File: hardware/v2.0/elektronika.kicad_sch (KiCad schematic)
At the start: 42 parts, among them J1 Conn_02x06_Odd_Even, J12 Conn_01x02, J2 Micro_SD_Card, J3 Conn_01x06, Q4 Q_NMOS_GSD, Q5 Q_PMOS_GSD, Q6 Q_NMOS_GSD, Q7 Q_NMOS_GSD, Q8 Q_NMOS_GSD

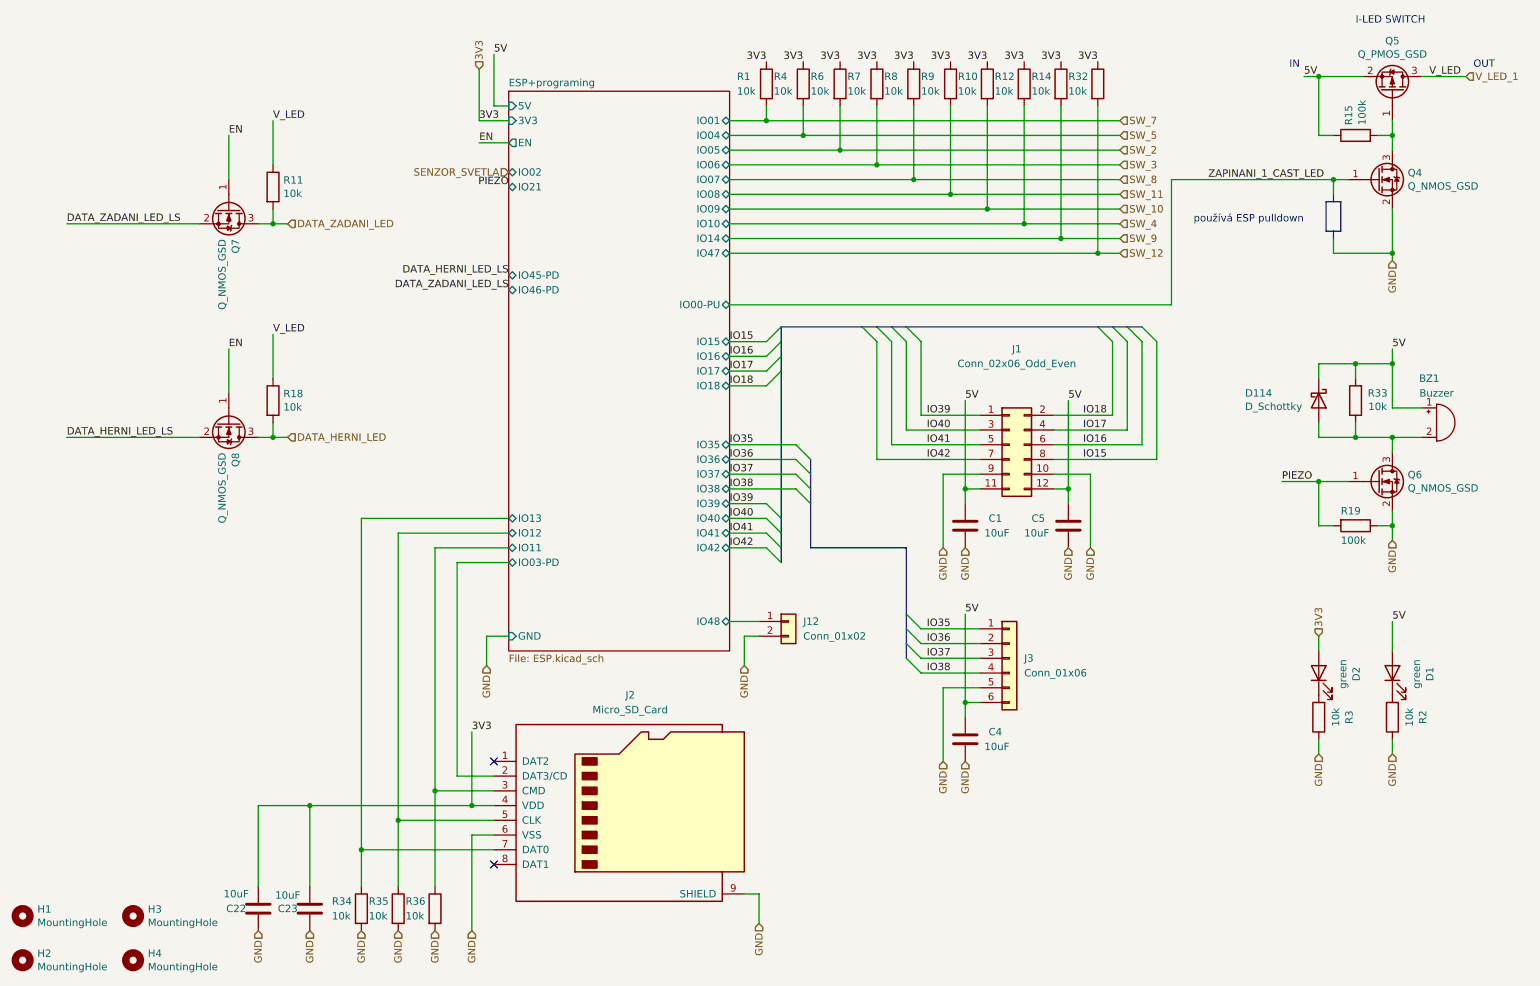
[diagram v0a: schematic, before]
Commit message: RH v2 version
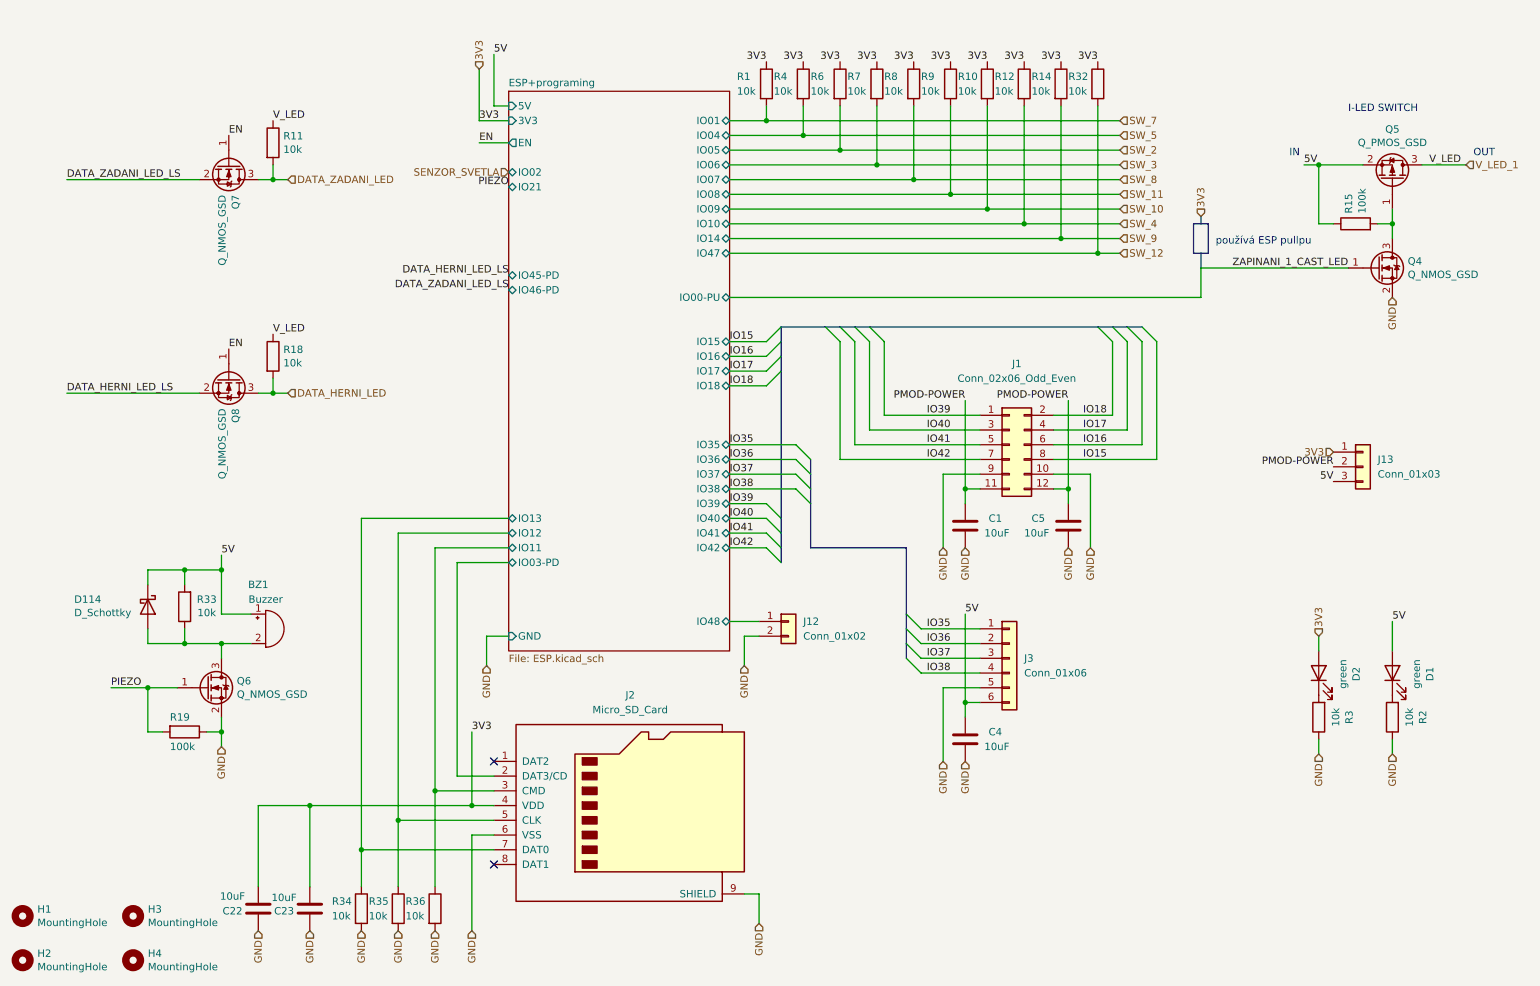
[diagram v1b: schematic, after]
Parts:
- added J13: Conn_01x03, Connector_PinHeader_2.54mm:PinHeader_1x03_P2.54mm_Horizontal, symbol Connector_Generic:Conn_01x03
- BZ1: footprint my_library:PIEZO -> Robotarna_KiCad_Library:ELKS-PIEZO; LCSC C3015481 -> C201041
- J1: JLCPCB_CORRECTION (none) -> -1.27;6.35;270; LCSC (none) -> C2897426
- J12, J3: JLCPCB_IGNORE (none) -> 1
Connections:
- net 3V3: now also J13.1 (Pin_1)
- net 5V: now also J13.3 (Pin_3); no longer C1.1, C5.1, J1.11 (Pin_11), J1.12 (Pin_12)
- new net PMOD-POWER: C1.1, C5.1, J1.11 (Pin_11), J1.12 (Pin_12), J13.2 (Pin_2)
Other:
- note added: "používá ESP pullpu"
- note removed: "používá ESP pulldown"
- moved on the sheet: BZ1, D114, Q6, Q7, Q8, R11, R18, R19, R33
